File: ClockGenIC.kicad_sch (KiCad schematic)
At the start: 9 parts, among them J5 Conn_Coaxial, U1 ADF4351, U4 ADF4351BCPZ-RL7

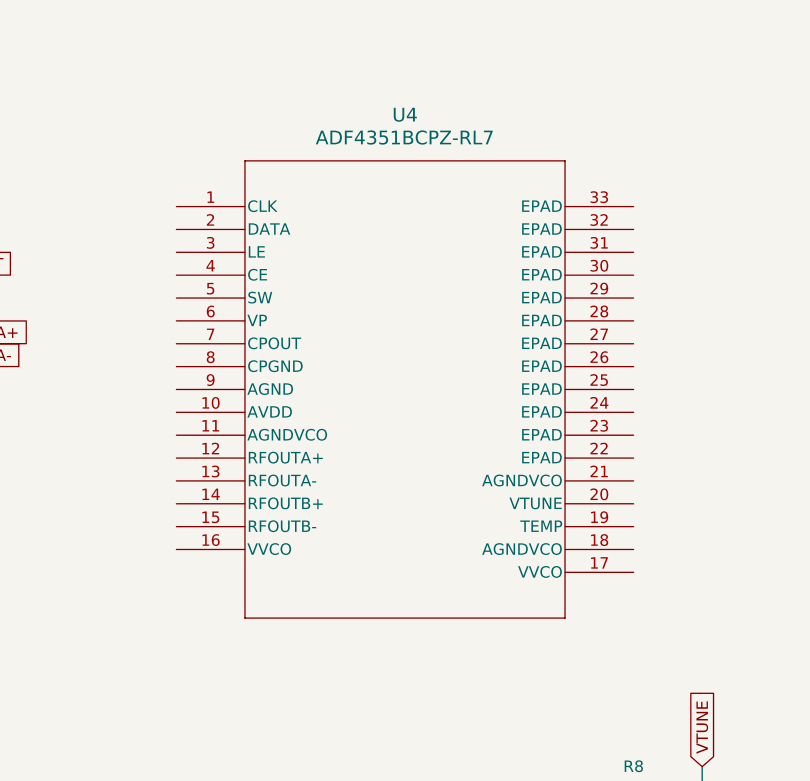
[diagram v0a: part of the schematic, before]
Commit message: updated schematic
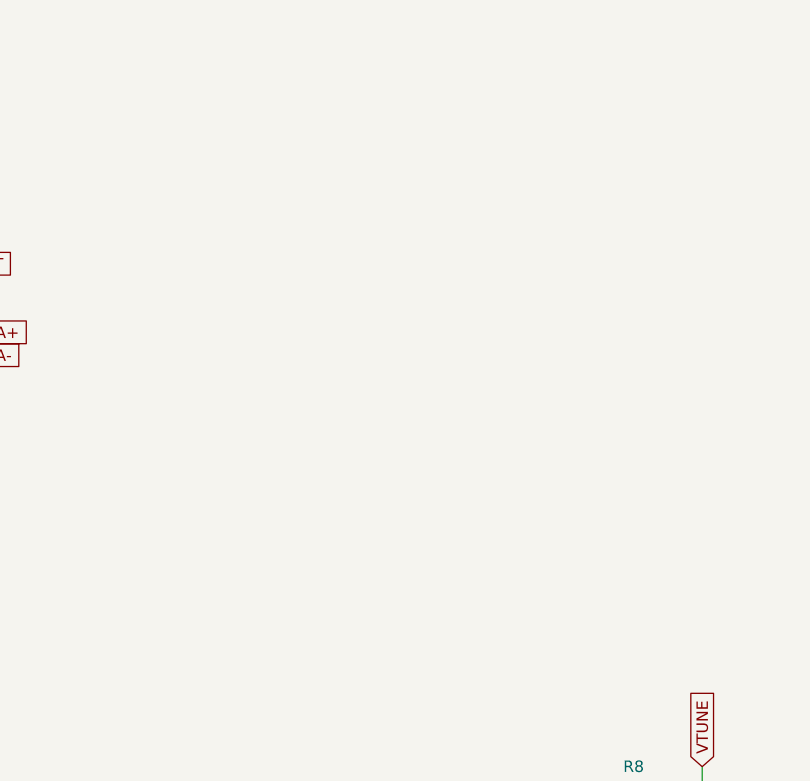
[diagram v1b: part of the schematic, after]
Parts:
- removed U4: ADF4351BCPZ-RL7, CP_32_7_ADI, symbol ADF4351BCPZ-RL7:ADF4351BCPZ-RL7
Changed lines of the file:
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@@
-	)
-	(symbol
-		(lib_id "ADF4351BCPZ-RL7:ADF4351BCPZ-RL7")
-		(at 176.53 59.69 0)
-		(unit 1)
-		(exclude_from_sim no)
-		(in_bom yes)
-		(on_board yes)
-		(dnp no)
-		(fields_autoplaced yes)
-		(property "Reference" "U4"
-			(at 201.93 49.53 0)
-			(effects
-				(font
-					(size 1.524 1.524)
-				)
-			)
-		)
-		(property "Value" "ADF4351BCPZ-RL7"
-			(at 201.93 52.07 0)
-			(effects
-				(font
-					(size 1.524 1.524)
-				)
-			)
-		)
-		(property "Footprint" "CP_32_7_ADI"
-			(at 176.53 59.69 0)
-			(effects
-				(font
-					(size 1.27 1.27)
-					(italic yes)
-				)
-				(hide yes)
-			)
-		)
-		(property "Datasheet" "https://www.analog.com/media/en/technical-documentation/data-sheets/ADF4351.pdf"
-			(at 176.53 59.69 0)
-			(effects
-				(font
-					(size 1.27 1.27)
-					(italic yes)
-				)
-				(hide yes)
-			)
-		)
-		(property "Description" ""
-			(at 176.53 59.69 0)
-			(effects
-				(font
-					(size 1.27 1.27)
-				)
-				(hide yes)
-			)
-		)
-		(pin "1"
-		)
-		(pin "14"
-		)
-		(pin "2"
-		)
-		(pin "4"
-		)
-		(pin "9"
-		)
-		(pin "10"
-		)
-		(pin "11"
-		)
-		(pin "3"
-		)
-		(pin "5"
-		)
-		(pin "12"
-		)
-		(pin "13"
-		)
-		(pin "7"
-		)
-		(pin "6"
-		)
-		(pin "8"
-		)
-		(pin "33"
-		)
-		(pin "32"
-		)
-		(pin "29"
-		)
-		(pin "15"
-		)
-		(pin "27"
-		)
-		(pin "26"
-		)
-		(pin "30"
-		)
-		(pin "24"
-		)
-		(pin "28"
-		)
-		(pin "16"
-		)
-		(pin "25"
-		)
-		(pin "22"
-		)
-		(pin "23"
-		)
-		(pin "21"
-		)
-		(pin "31"
-		)
-		(pin "20"
-		)
-		(pin "19"
-		)
-		(pin "17"
-		)
-		(pin "18"
-		)
-		(instances
-			(project ""
-				(path "/e1444a2d-a0c4-493c-a136-c624dc084e46/5eadf96c-4633-4d78-8a47-09b3347a9db0"
-					(reference "U4")
-					(unit 1)
-				)
-			)
-		)
 	)
 	(symbol
